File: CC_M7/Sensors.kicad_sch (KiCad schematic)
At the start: 12 parts, among them U2 BMI088, U3 BMP388, U4 BMM150, U5 24AA64T-I/OT

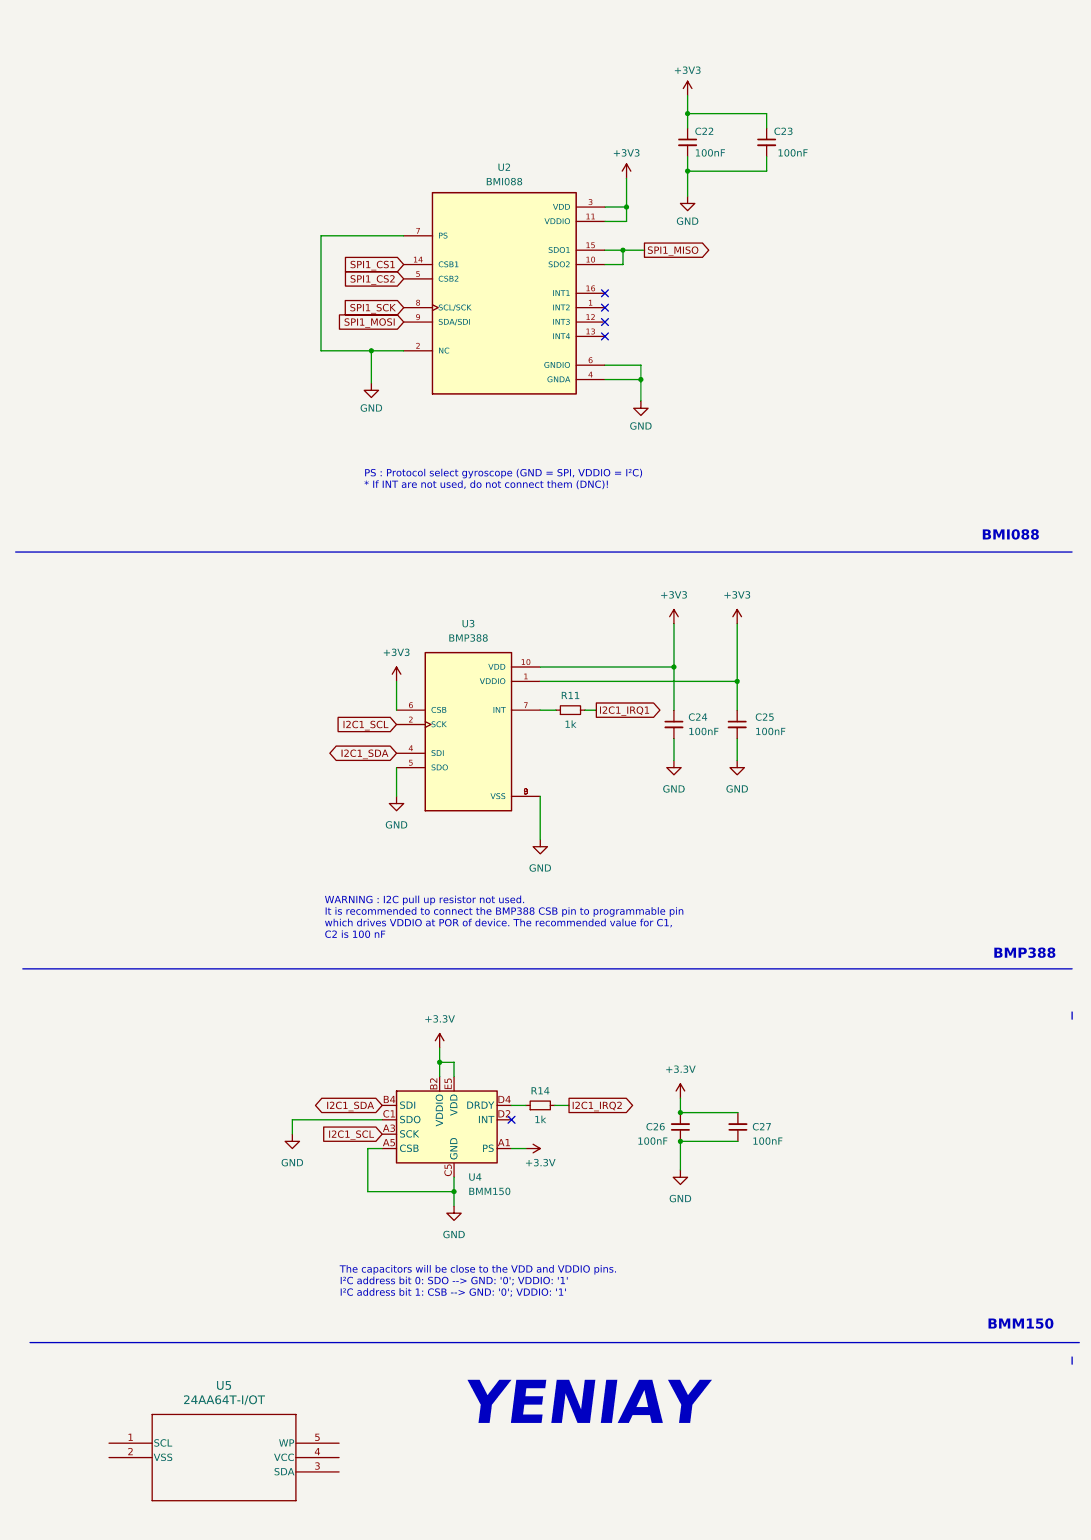
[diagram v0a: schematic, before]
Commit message: EEPROM
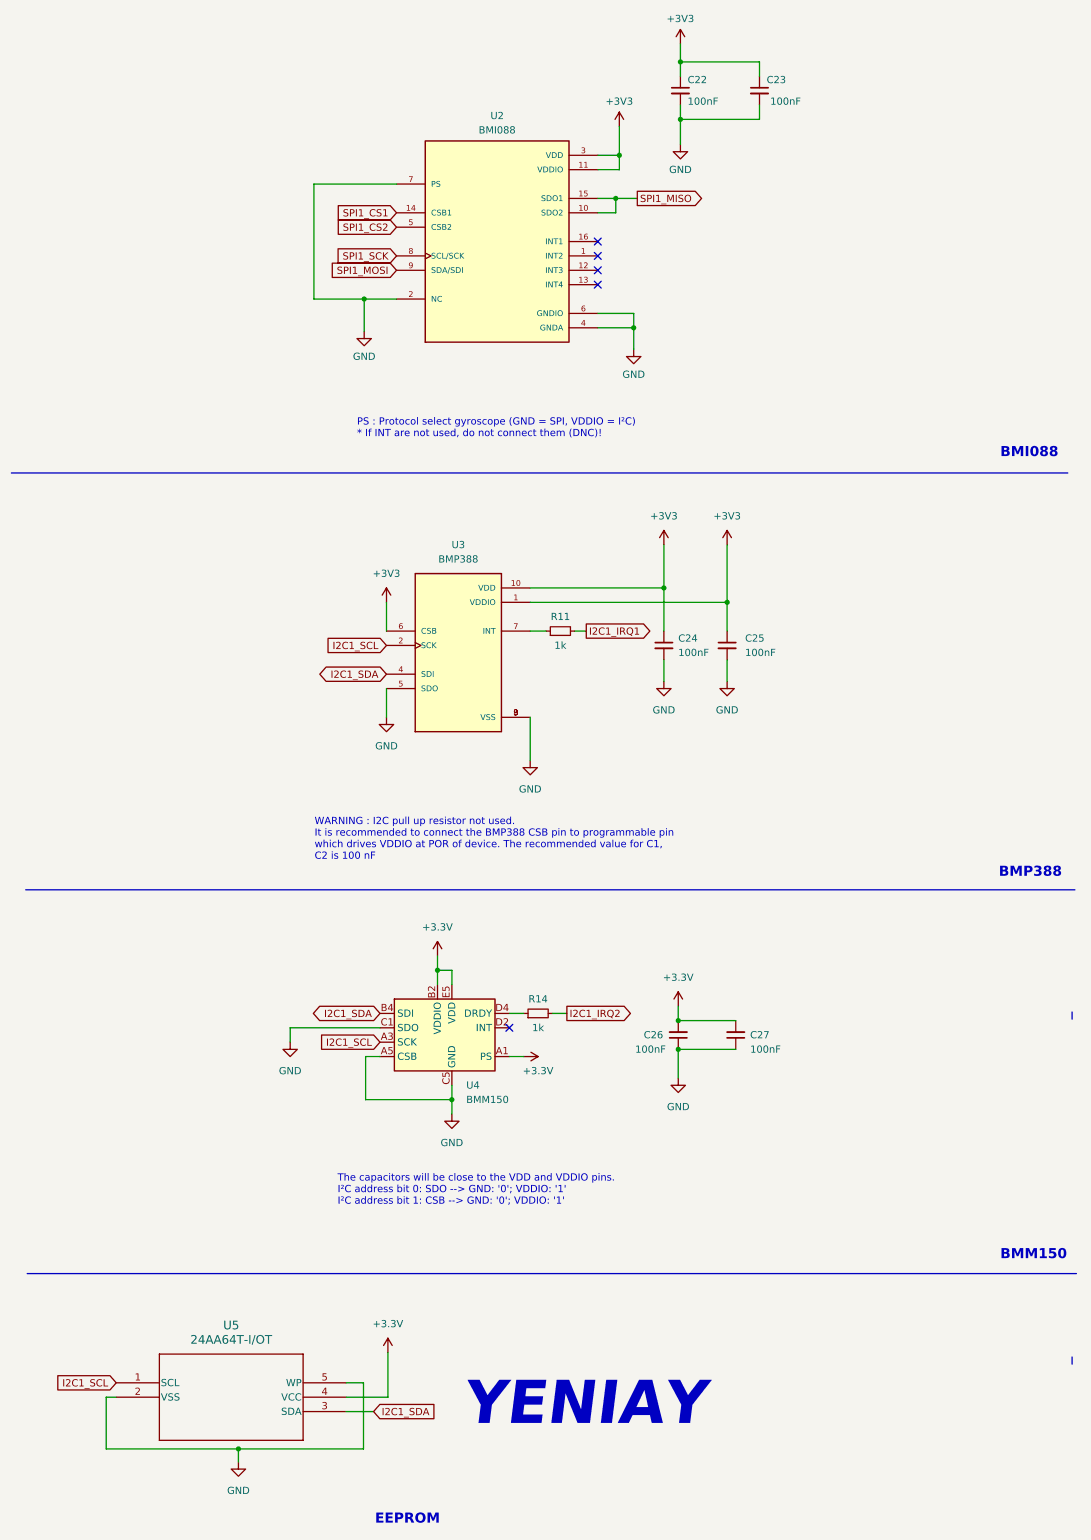
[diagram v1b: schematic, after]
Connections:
- net +3.3V: now also U5.4 (VCC)
- net GND: now also U5.2 (VSS), U5.5 (WP)
- net I2C1_SCL: now also U5.1 (SCL)
- net I2C1_SDA: now also U5.3 (SDA)
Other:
- note added: "EEPROM"
- moved on the sheet: C22, C23, C24, C25, C26, C27, R11, R14, U2, U3, U4, U5
